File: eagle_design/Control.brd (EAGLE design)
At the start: 55.9 x 63.2 mm, 17 parts, among them K1 G5LE, K2 G5LE, K3 G5LE

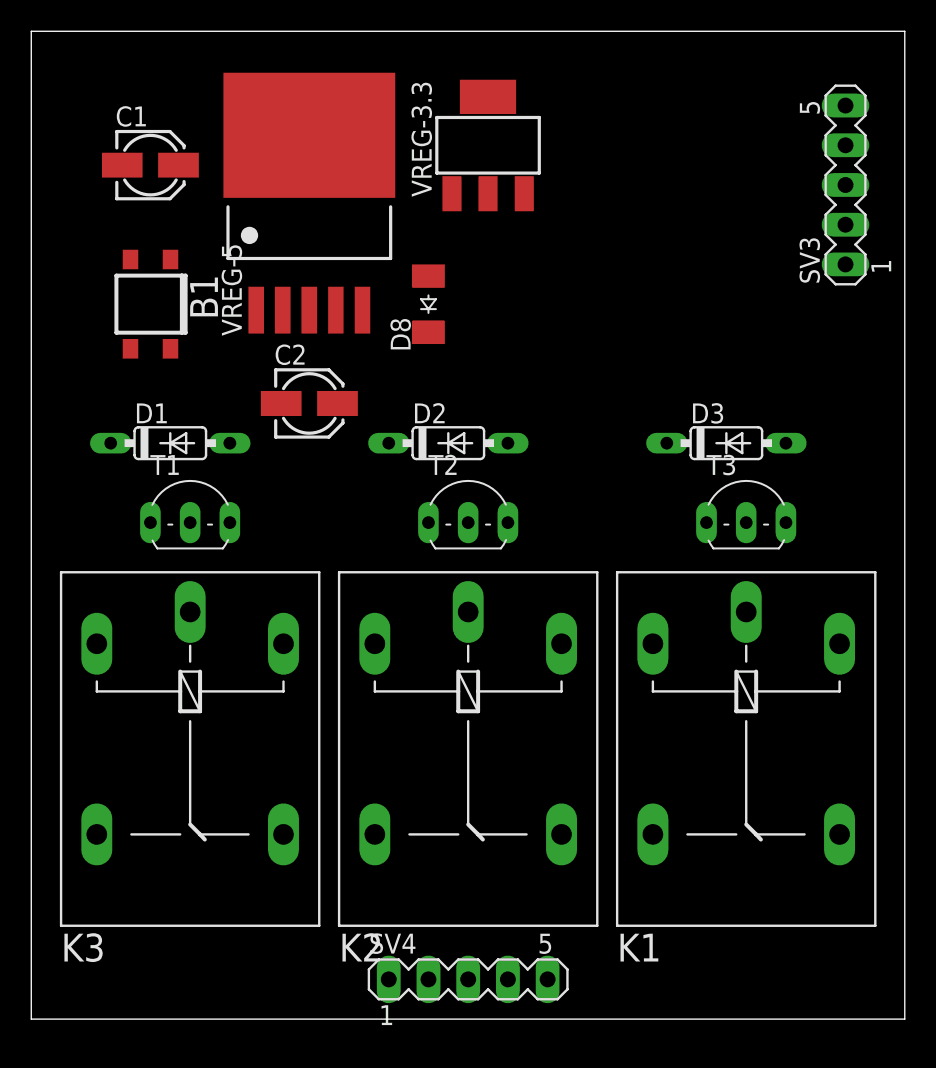
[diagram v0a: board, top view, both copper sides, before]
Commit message: Did some more PCB design and added some datasheets
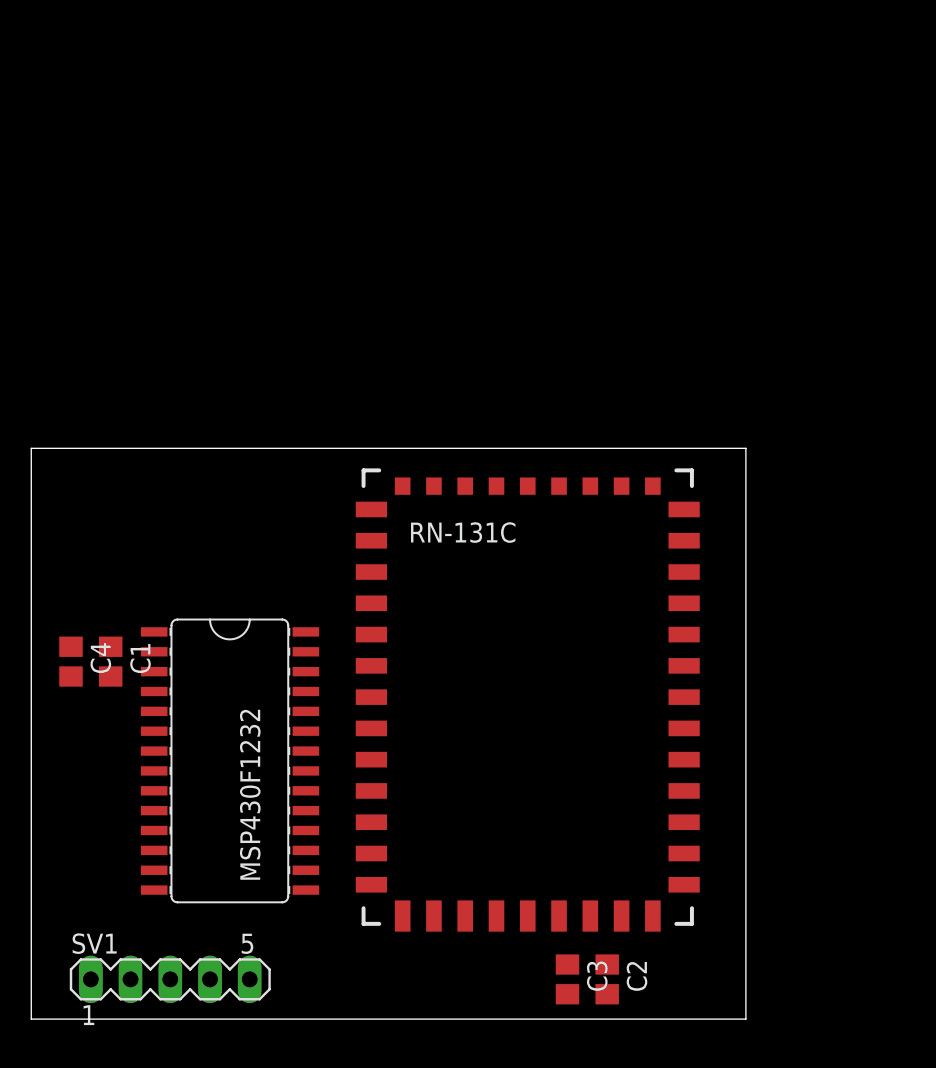
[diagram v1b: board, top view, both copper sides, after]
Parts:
- removed B1: RECTIFIER-S80, rectifier:TO-269AA
- removed D1, D2, D3: 1N4148DO35-7, diode:DO35-7
- removed D8: CGRM4001-G, diode:SOD-123_MINI-SMA
- removed K1, K2, K3: G5LE, relay:G5LE
- removed SV3, SV4: (no value), con-lstb:MA05-1
- removed T1, T2, T3: (no value), transistor-neu-to92:TO92-EBC
- removed VREG-3.3: (no value), linear-technology:SOT223
- removed VREG-5: TL2575-05, texas:TO-263-5
- added C3, C4: 10uF, rcl:C0805
- added MSP430F1232: F12X2---DW28, TI_MSP430_v16:DW28
- added RN-131C: RN-131G, SparkFun:RN-131G
- added SV1: (no value), con-lstb:MA05-1
- C1: value 100uF -> 0.1uF; device rcl:153CLV-0405 -> rcl:C0805
- C2: value 330uF -> 0.1uF; device rcl:153CLV-0405 -> rcl:C0805
- moved C2 41.5 mm to (36.8, 2.54), turned to 270 degrees
- moved C1 31.9 mm to (5.08, 22.9), turned to 270 degrees
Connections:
- removed net 3.3+: SV3.5, VREG-3.3.3
- removed net 5V+: C2.+, D1.C, D2.C, D3.C, K1.1, K2.1, K3.1, VREG-3.3.1, VREG-5.4
- removed net G: K3.S, SV4.1
- removed net N$1: B1.+, C1.+, VREG-5.1
- removed net N$2: D1.A, K3.2, T1.C
- removed net N$3: D2.A, K2.2, T2.C
- removed net N$4: D8.C, VREG-5.2
- removed net N$5: D3.A, K1.2, T3.C
- removed net N$6: K1.O
- removed net N$7: K2.O
- removed net N$8: K3.O
- removed net VAC+: B1.AC1, K1.P, K2.P, K3.P, SV4.5
- removed net VAC-: SV4.4
- removed net W: K1.S, SV4.3
- removed net Y: K2.S, SV4.2
- new net RESET: RN-131C.RESET
- new net RN-RX: MSP430F1232.15, RN-131C.UART-RX
- new net RN-TX: MSP430F1232.16, RN-131C.UART-TX
- new net VCC: C1.1, C2.1, C3.1, C4.1, MSP430F1232.2, RN-131C.VDD-BATT, RN-131C.VDD-IN, SV1.5
- net AC: now also SV1.2; no longer SV3.2, T2.B
- net FAN: now also SV1.1; no longer SV3.1, T1.B
- net GND: now also C1.2, C2.2, C3.2, C4.2, MSP430F1232.4, RN-131C.3.3-RIN, RN-131C.GND0, RN-131C.GND1, RN-131C.GND2, RN-131C.GND3, RN-131C.GND4, RN-131C.GND5, RN-131C.GND6, RN-131C.GND7, RN-131C.GND8, RN-131C.GND9, SV1.4; no longer B1.-, C1.-, C2.-, D8.A, SV3.4, T1.E, T2.E, T3.E, VREG-3.3.2, VREG-3.3.4, VREG-5.3, VREG-5.5, VREG-5.TAB
- net HEAT: now also SV1.3; no longer SV3.3, T3.B
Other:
- board size 55.9 x 63.2 mm -> 45.7 x 36.5 mm
